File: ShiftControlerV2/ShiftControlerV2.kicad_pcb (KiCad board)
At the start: 2 copper layers, 33 parts, among them J1 Conn_02x06_Counter_Clockwise, Q1 BTN8982TA, Q2 BTN8982TA, Q3 BSS138, Q4 BSS138, U1 ControllerBoardV2, U2 NCV7805BDTRKG

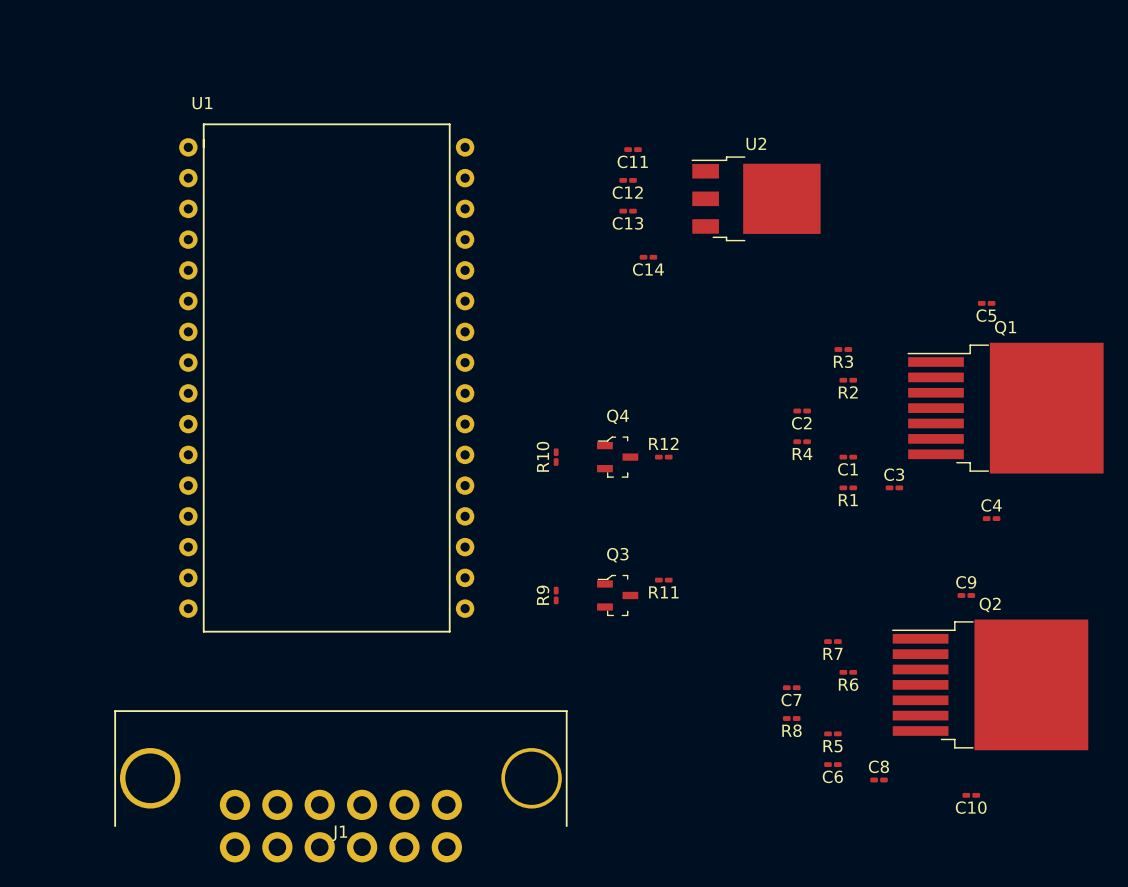
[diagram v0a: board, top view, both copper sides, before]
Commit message: Schematic Revised
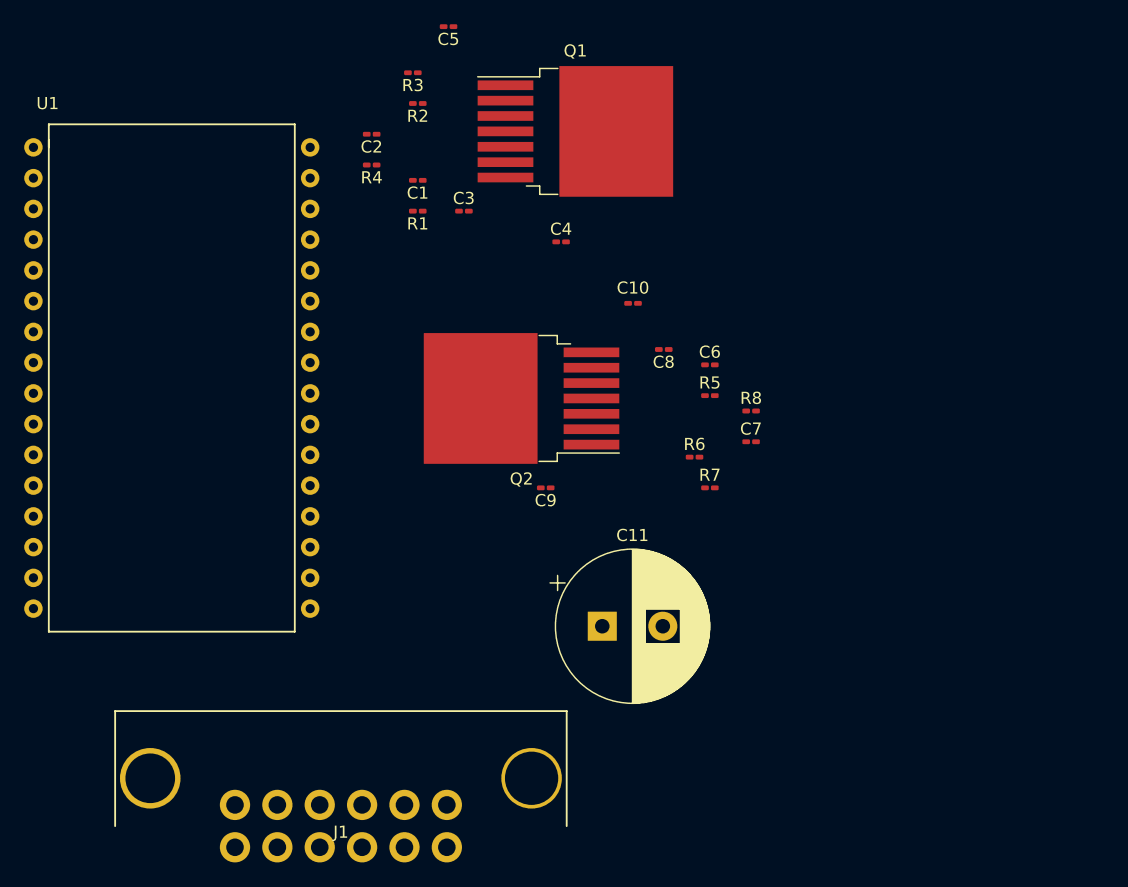
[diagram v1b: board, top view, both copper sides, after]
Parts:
- removed C12, C13: 10n, Capacitor_SMD:C_0201_0603Metric_Pad0.64x0.40mm_HandSolder
- removed C14: 10u, Capacitor_SMD:C_0201_0603Metric_Pad0.64x0.40mm_HandSolder
- removed Q3, Q4: BSS138, digikey-footprints:SOT-23-3
- removed R10, R11, R12, R9: 10k, Resistor_SMD:R_0201_0603Metric_Pad0.64x0.40mm_HandSolder
- removed U2: NCV7805BDTRKG, Package_TO_SOT_SMD:TO-252-3_TabPin4
- C11: value 10u -> 1000u; footprint Capacitor_SMD:C_0201_0603Metric_Pad0.64x0.40mm_HandSolder -> Capacitor_THT:CP_Radial_D12.5mm_P5.00mm
- moved C5 50.0 mm to (100.3, 41.9)
- moved C10 49.3 mm to (115.6, 64.8), turned to 0 degrees
- moved Q2 45.4 mm to (106.4, 72.6), turned to 180 degrees
- moved C3 42.3 mm to (101.6, 57.1)
- moved C4 42.3 mm to (109.6, 59.7)
- moved Q1 42.3 mm to (110.8, 50.6)
- moved R3 42.3 mm to (97.4, 45.7)
- moved R1 42.3 mm to (97.8, 57.1)
- moved R2 42.3 mm to (97.8, 48.3)
- moved C1 42.3 mm to (97.8, 54.6)
- moved C2 42.3 mm to (94.0, 50.8)
- moved R4 42.3 mm to (94.0, 53.3)
- moved C8 39.8 mm to (118.1, 68.6), turned to 180 degrees
- moved C11 39.5 mm to (113.0, 91.4), turned to 0 degrees
- moved C9 35.9 mm to (108.4, 80.0), turned to 180 degrees
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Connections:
- net Net-(U1-Pad24) renamed CURRENT1
- net Net-(U1-Pad25) renamed CURRENT2
- J1 pad 7: Net-(J1-Pad7) -> UARTTX
- J1 pad 8: Net-(J1-Pad8) -> UARTRX
- R2 pad 2: +5V -> INH1
- R6 pad 2: +5V -> INH2
- U1 pad 17: Net-(U1-Pad17) -> CANL
- U1 pad 18: Net-(U1-Pad18) -> CANH
- U1 pad 22: Net-(U1-Pad22) -> UARTRX
- U1 pad 23: Net-(U1-Pad23) -> UARTTX
- U1 pad 28: Net-(U1-Pad28) -> INH2
- U1 pad 29: Net-(U1-Pad29) -> INH1
